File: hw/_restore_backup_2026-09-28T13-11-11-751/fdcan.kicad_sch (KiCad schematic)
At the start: 2 parts, among them U3 AS5047D

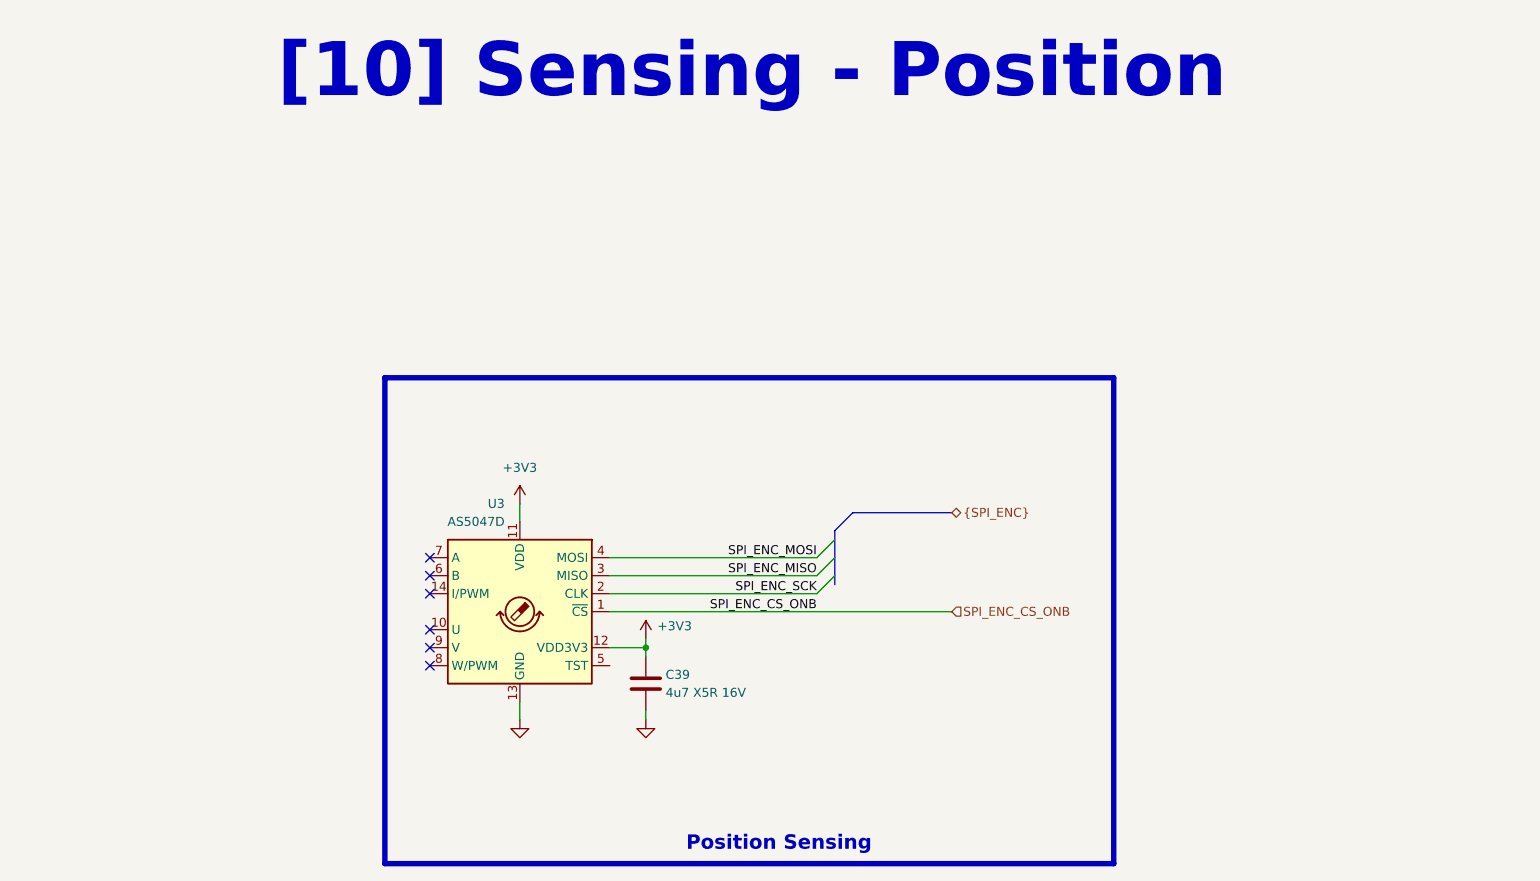
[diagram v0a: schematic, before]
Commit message: extended lcsc number coverage
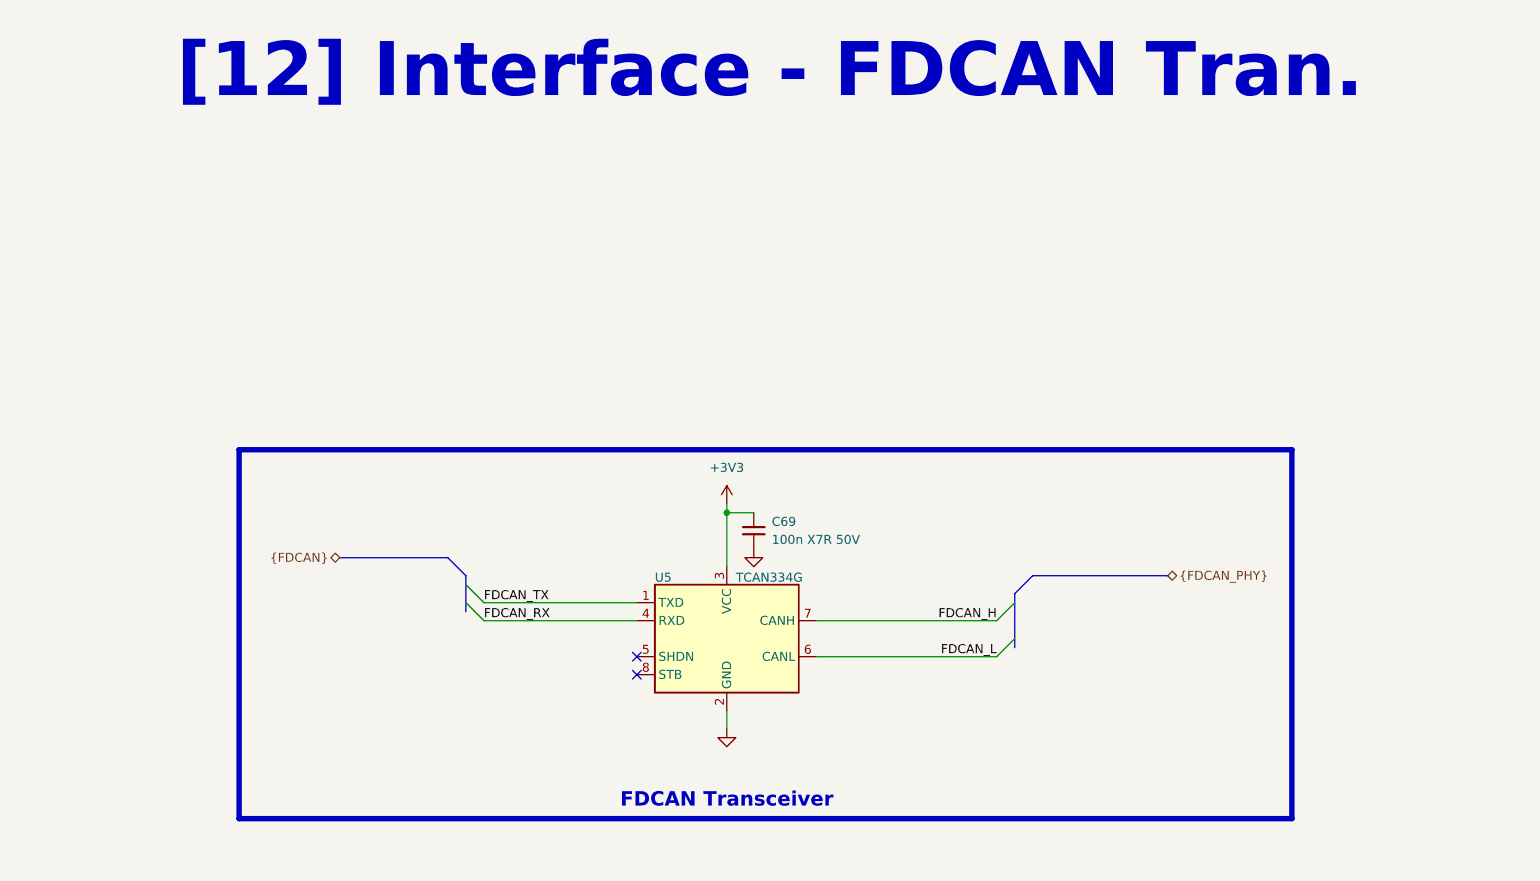
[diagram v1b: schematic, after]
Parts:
- removed C39: 4u7 X5R 16V, Capacitor_SMD:C_0603_1608Metric, symbol Device:C
- removed U3: AS5047D, Package_SO:TSSOP-14_4.4x5mm_P0.65mm, symbol Sensor_Magnetic:AS5047D
- added C69: 100n X7R 50V, Capacitor_SMD:C_0603_1608Metric, symbol Device:C_Small
- added U5: TCAN334G, Package_SO:TSSOP-14_4.4x5mm_P0.65mm, symbol Interface_CAN_LIN:TCAN334G
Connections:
- net +3V3: now also C69.1, U5.3 (VCC)
- net GND: now also C69.2, U5.2 (GND)
- new net FDCAN_H: U5.7 (CANH)
- new net FDCAN_L: U5.6 (CANL)
- new net FDCAN_RX: U5.4 (RXD)
- new net FDCAN_TX: U5.1 (TXD)
- no-connect marks 6 -> 2
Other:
- note added: "FDCAN Transceiver"
- note added: "[12] Interface - FDCAN Tran."
- note removed: "Position Sensing"
- note removed: "[10] Sensing - Position"
